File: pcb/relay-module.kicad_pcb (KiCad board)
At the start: 4 copper layers, 50 x 50 mm, 43 parts, among them J1 AVR-UPDI-6, J2 QWICC, J3 Power, K1 PR24-5V-900-1A, P1 MountingHole_Pad, P2 MountingHole_Pad, P3 MountingHole_Pad, P4 MountingHole_Pad, Q1 MMBT3904, U2 ATtiny1616-M, U3 LTV-356T

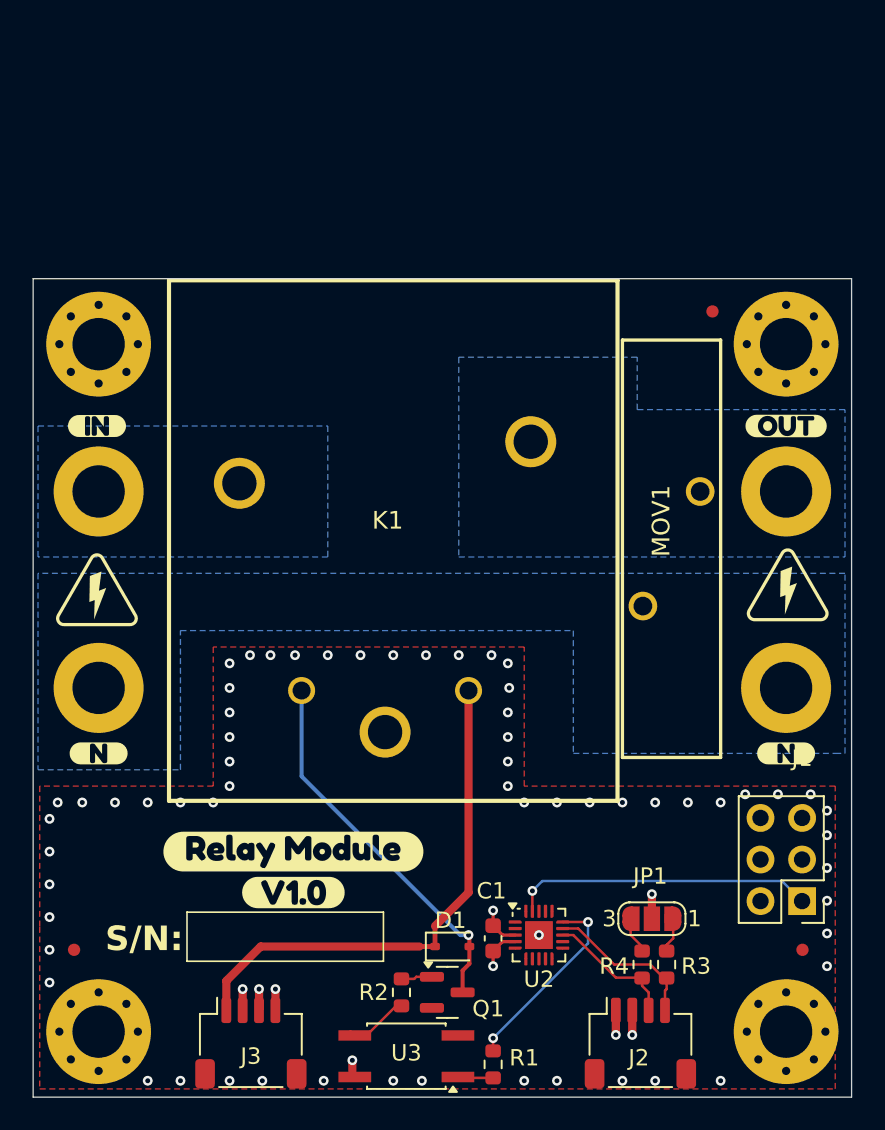
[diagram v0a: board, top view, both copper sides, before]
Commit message: v1.0 Relay Module Panel 2x2
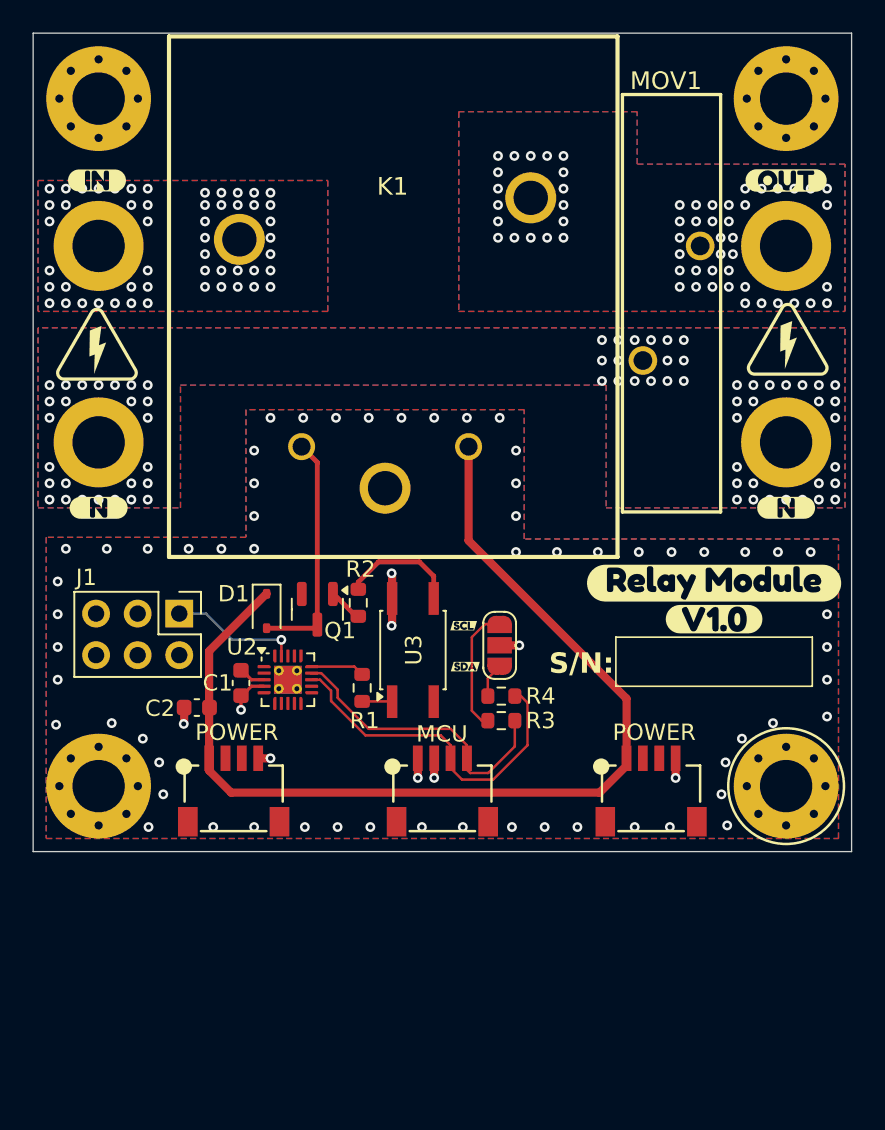
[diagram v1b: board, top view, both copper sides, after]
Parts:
- removed FID1, FID2, FID3: Fiducial, Fiducial:Fiducial_0.75mm_Mask1.5mm
- removed kibuzzard-67F88791: G***, kibuzzard-67F88791
- removed kibuzzard-67F88799: G***, kibuzzard-67F88799
- removed kibuzzard-67F8886E: G***, kibuzzard-67F8886E
- removed kibuzzard-67F88877: G***, kibuzzard-67F88877
- added C2: .1uF, Capacitor_SMD:C_0603_1608Metric, F.Cu at (60.0, 141.2)
- added J4: Power Out, CRGM Connector:SM04B-SRSS-TB, F.Cu at (62.2, 144.3)
- added kibuzzard-6801052A: G***, kibuzzard-6801052A, F.Cu at (91.6, 133.6)
- added kibuzzard-6801053F: G***, kibuzzard-6801053F, F.Cu at (91.6, 135.8)
- added kibuzzard-6801AC5F: G***, kibuzzard-6801AC5F, F.Cu at (76.3, 136.2)
- added kibuzzard-6801ACAF: G***, kibuzzard-6801ACAF, F.Cu at (76.4, 138.7)
- added kibuzzard-6802999E: G***, kibuzzard-6802999E, B.Cu at (75.0, 120.8)
- added kibuzzard-68029C11: G***, kibuzzard-68029C11, B.Cu at (75.0, 117.6)
- J2: footprint Connector_JST:JST_SH_SM04B-SRSS-TB_1x04-1MP_P1.00mm_Horizontal -> CRGM Connector:SM04B-SRSS-TB
- J3: value Power -> Power In; footprint Connector_JST:JST_SH_SM04B-SRSS-TB_1x04-1MP_P1.00mm_Horizontal -> CRGM Connector:SM04B-SRSS-TB
- LOGO1: footprint CRGM Logos:Aquarius Logo 10mm -> CRGM Logos:Aquarius Logo 5mm
- LOGO3: footprint CRGM Logos:FNWW Face 10mm -> CRGM Logos:FNWW Face 5mm
- U2: footprint Package_DFN_QFN:VQFN-20-1EP_3x3mm_P0.4mm_EP1.7x1.7mm -> CRG Makes:VQFN-20-1EP_3x3mm_P0.4mm_EP1.7x1.7mm_ThermalVias
- moved J1 41.9 mm to (58.9, 135.5), turned to -90 degrees
- moved LOGO1 41.9 mm to (75.1, 113.2)
- moved J3 30.0 mm to (87.8, 144.3), turned to 180 degrees
- moved U3 24.8 mm to (73.2, 137.7), turned to 90 degrees
- moved Q1 24.7 mm to (67.4, 135.2), turned to -90 degrees
- moved R1 24.4 mm to (70.1, 140.0)
- moved R2 23.9 mm to (69.9, 134.8), turned to -90 degrees
- moved D1 23.4 mm to (64.3, 135.3), turned to -90 degrees
- moved LOGO5 22.1 mm to (70.2, 144.2)
- moved C1 21.9 mm to (62.7, 139.7)
- moved U2 21.9 mm to (65.6, 139.5)
- moved J2 21.2 mm to (75.0, 144.3), turned to 180 degrees
- moved JP1 19.1 mm to (78.5, 137.4), turned to -90 degrees
- moved R4 18.5 mm to (78.6, 140.5), turned to 180 degrees
- moved R3 18.0 mm to (78.6, 142.0), turned to 180 degrees
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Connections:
- net /RELAY_CTRL renamed RELAY_CTRL
- net /UPDI renamed UPDI
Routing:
- net +5V: track 31.9 -> 62.5 mm
- net /SDA: track 8.08 -> 21.3 mm
- net UPDI: track 18.5 -> 7.89 mm
- net /SCL: track 9.65 -> 18.4 mm
- net /RELAY_CONTROL: track 23.1 -> 14.5 mm, vias 1 -> 0
- net RELAY_CTRL: track 11.8 -> 3.28 mm, vias 2 -> 0
- net Net-(JP1-A): track 2.14 -> 7.75 mm
- net Net-(R2-Pad1): track 3.95 -> 7.29 mm
- net GND: track 6.61 -> 3.98 mm, vias 66 -> 63
- net +3.3V: track 7.90 -> 10.2 mm, vias 5 -> 7
- net Net-(R1-Pad2): track 2.35 -> 1.84 mm
- net /NEUTRAL: vias 0 -> 68
- net /LOAD_OUT: vias 0 -> 56
- net /LOAD_IN: vias 0 -> 52
- added copper zone on F.Cu, net /LOAD_IN
- added copper zone on In1.Cu, net /LOAD_IN
- added copper zone on In2.Cu, net /LOAD_IN
- added copper zone on F.Cu, net /LOAD_OUT
- added copper zone on In1.Cu, net /LOAD_OUT
- added copper zone on In2.Cu, net /LOAD_OUT
- added copper zone on F.Cu, net /NEUTRAL
- added copper zone on In1.Cu, net /NEUTRAL
- added copper zone on In2.Cu, net /NEUTRAL
- added copper zone on B.Cu, net GND
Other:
- board text added: "MCU"
- board text added: "POWER"
- board text added: "Score Line"
